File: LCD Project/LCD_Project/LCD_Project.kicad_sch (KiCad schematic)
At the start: 6 parts, among them IC1 REG1117-5, J1 DT15-4P, U1 Teensy4.0

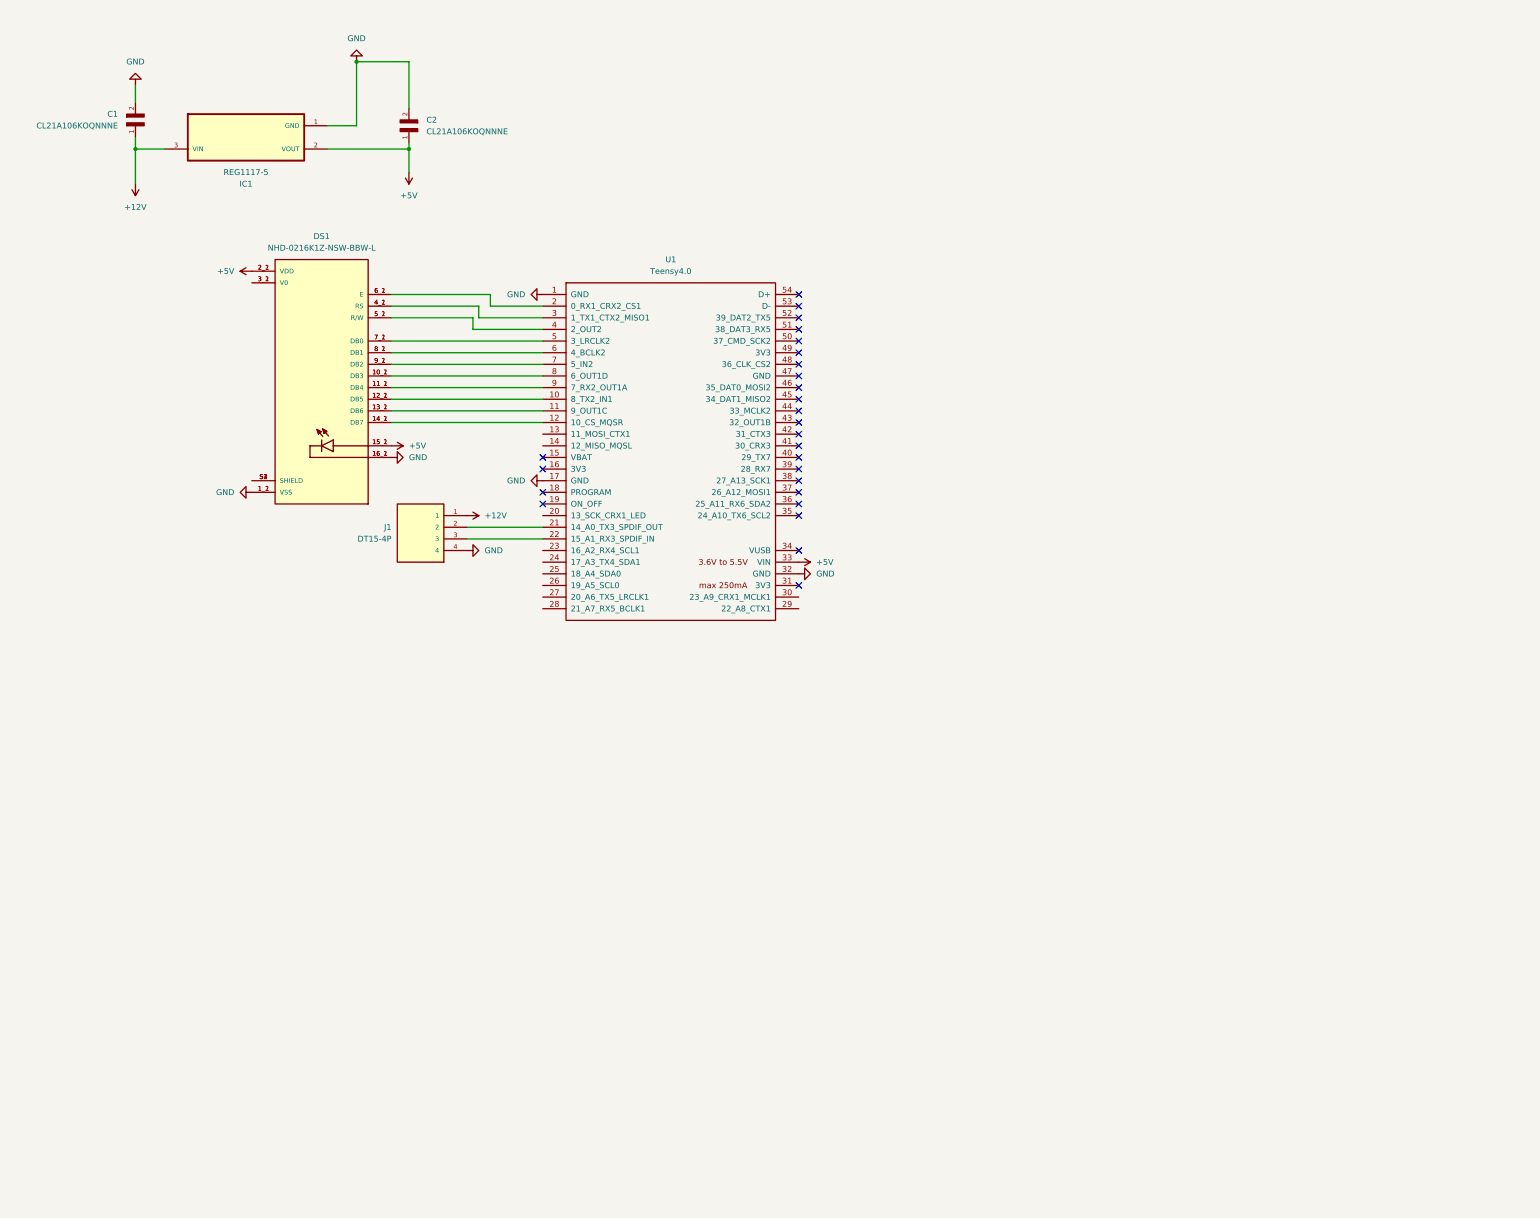
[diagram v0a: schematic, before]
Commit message: Add files via upload
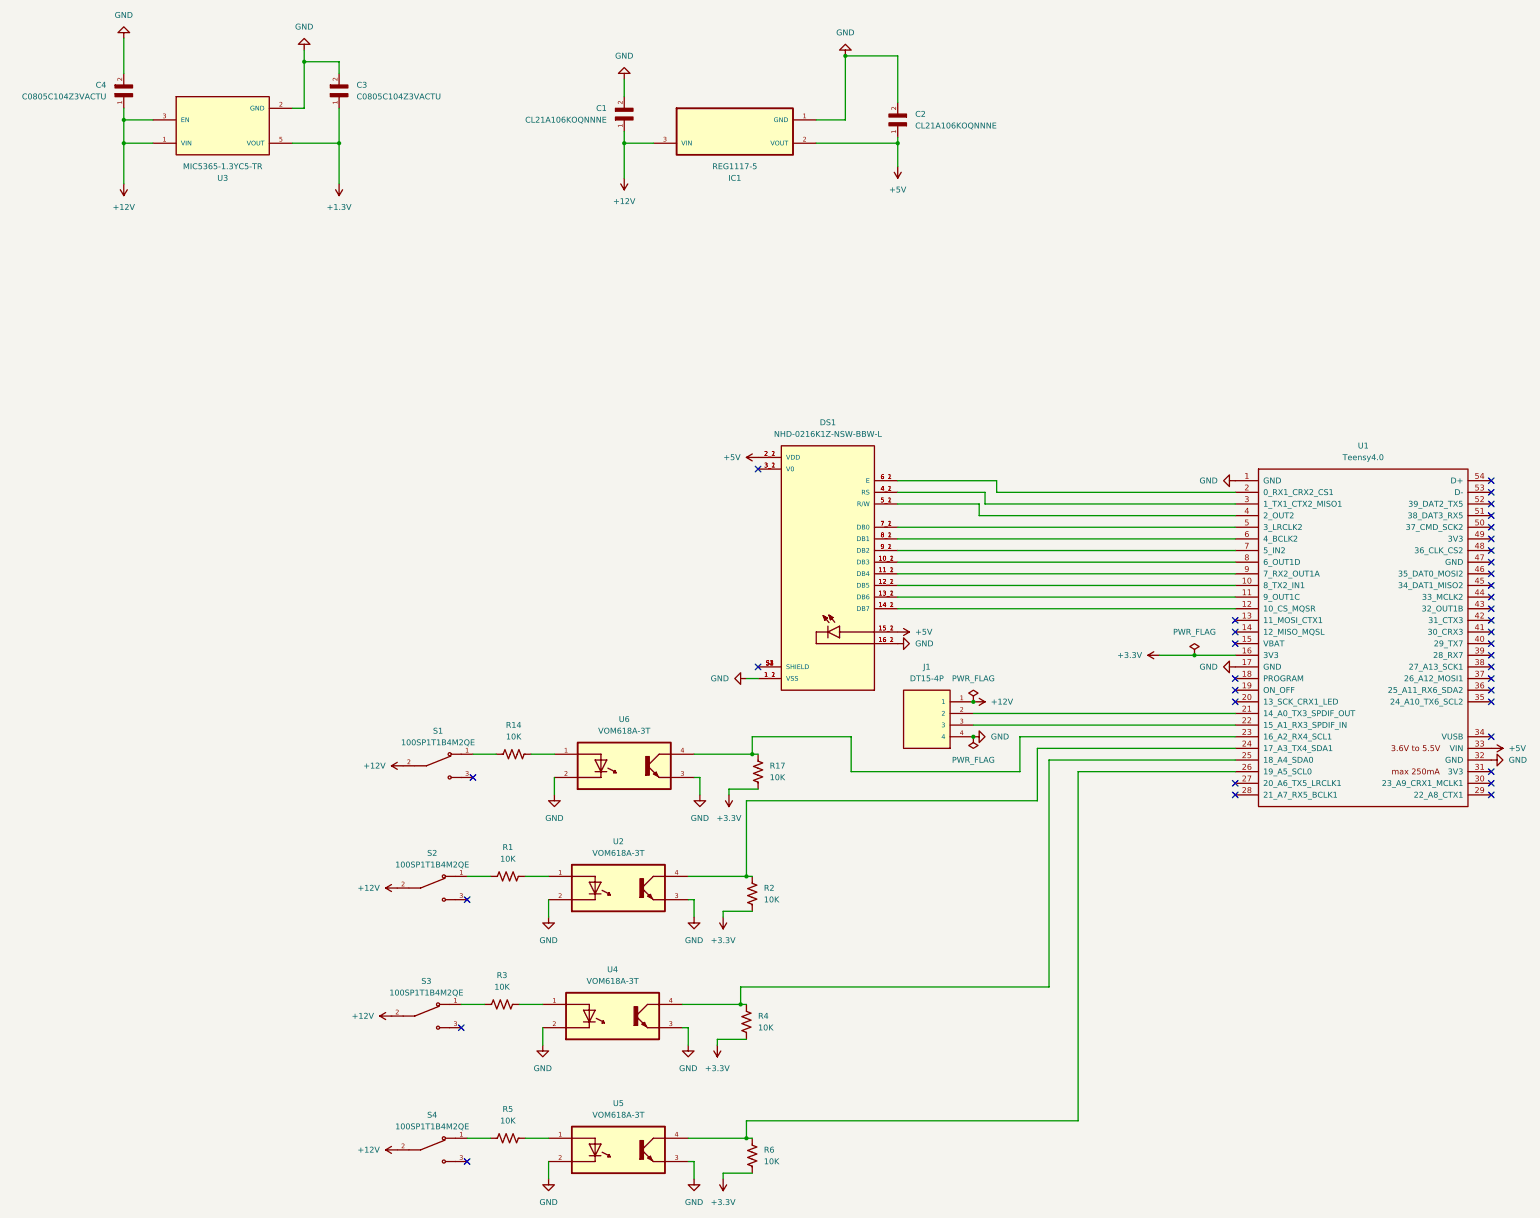
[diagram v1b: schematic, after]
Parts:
- added C3, C4: C0805C104Z3VACTU, C0805C104Z3VACTU:CAPC2012X88N, symbol C0805C104Z3VACTU:C0805C104Z3VACTU
- added R1, R14, R17, R2, R3, R4, R5, R6: 10K, symbol Device:R_US
- added S1, S2, S3, S4: 100SP1T1B4M2QE, 100SP1T1B4M2QE:SW_100SP1T1B4M2QE, symbol 100SP1T1B4M2QE:100SP1T1B4M2QE
- added U2, U4, U5, U6: VOM618A-3T, VOM618A-3T:SOIC254P695X242-4N, symbol VOM618A-3T:VOM618A-3T
- added U3: MIC5365-1.3YC5-TR, MIC5365-1.3YC5-TR:SOT65P210X110-5N, symbol MIC5365-1.3YC5-TR:MIC5365-1.3YC5-TR
- U1: footprint (none) -> teensy.pretty-master:Teensy40_SMT
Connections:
- net +12V: now also C4.1, S1.2, S2.2, S3.2, S4.2, U3.1 (VIN), U3.3 (EN)
- net GND: now also C3.2, C4.2, U2.2, U2.3, U3.2 (GND), U4.2, U4.3, U5.2, U5.3, U6.2, U6.3
- net +3.3V: now reaches U1.16 (3V3)
- net +3.3V: now also R17.2, R2.2, R4.2, R6.2
- net at U1.23 (16_A2_RX4_SCL1): now also R17.1, U6.4
- net at U1.24 (17_A3_TX4_SDA1): now also R2.1, U2.4
- net at U1.25 (18_A4_SDA0): now also R4.1, U4.4
- net at U1.26 (19_A5_SCL0): now also R6.1, U5.4
- new net: R3.1, S3.1
- new net: R3.2, U4.1
- new net: R14.1, S1.1
- new net: R1.1, S2.1
- new net: R5.1, S4.1
- new net: R14.2, U6.1
- new net: R1.2, U2.1
- new net: R5.2, U5.1
- new net +1.3V: C3.1, U3.5 (VOUT)
- no-connect marks 26 -> 38
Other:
- moved on the sheet: C1, C2, DS1, IC1, U1

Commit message: Add files via upload
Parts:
- R1, R14, R17, R2, R3, R4, R5, R6: footprint (none) -> CRCW08051K00FKEA:RESC2012X50N
